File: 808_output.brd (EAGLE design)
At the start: 100.6 x 80.6 mm, 31 parts, among them IC1 TL072P

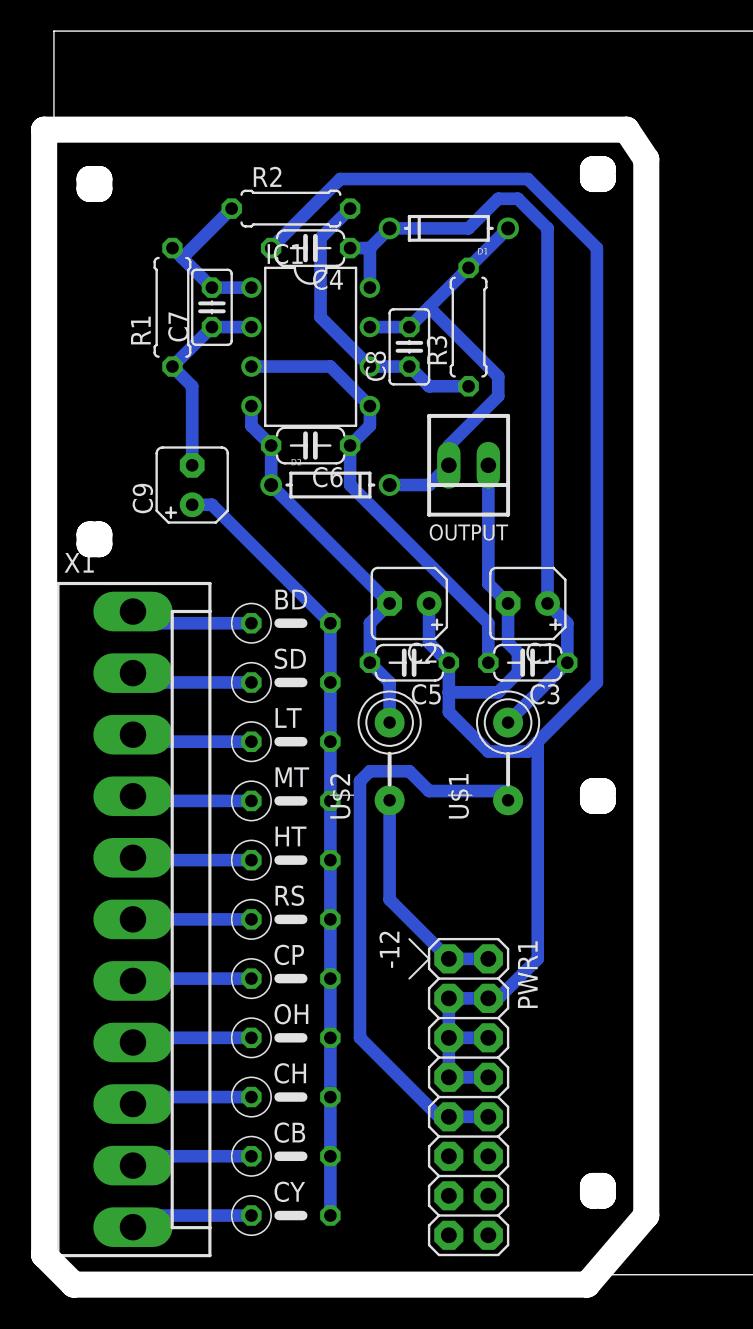
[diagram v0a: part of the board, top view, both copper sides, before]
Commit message: closer to og 808
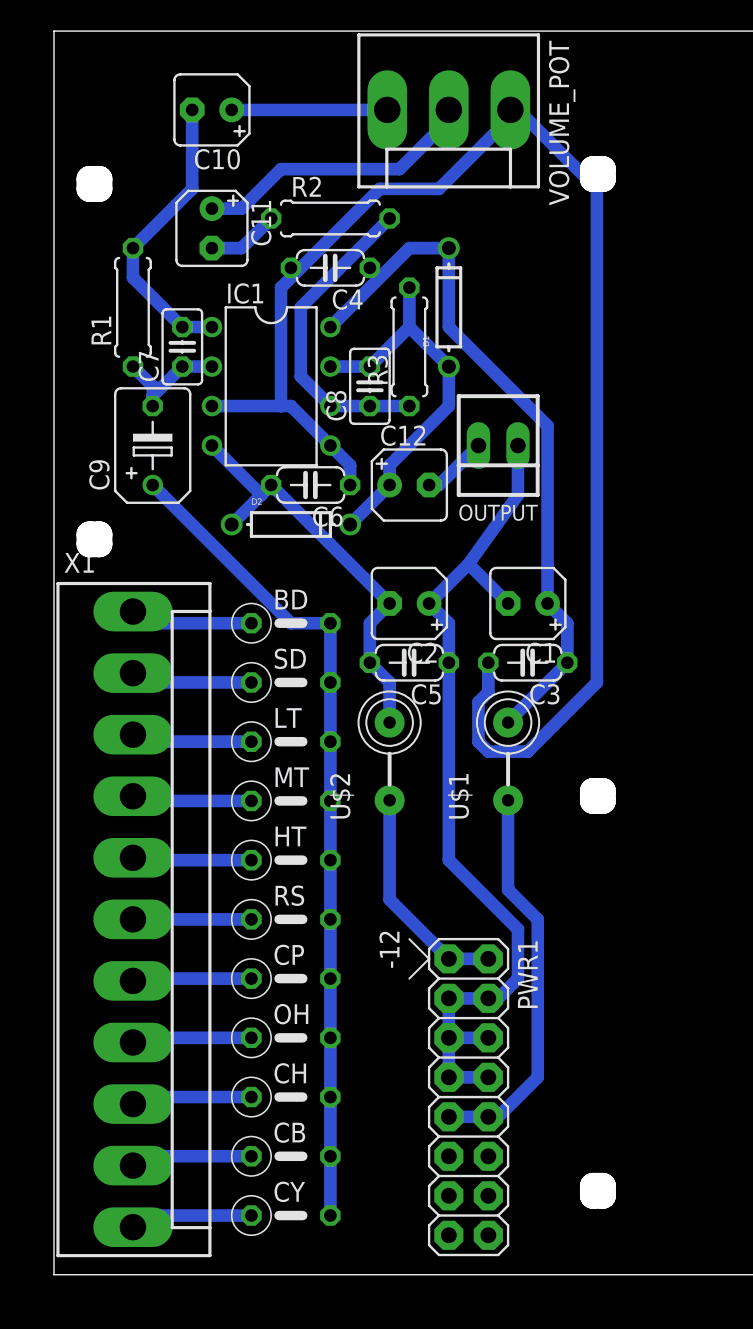
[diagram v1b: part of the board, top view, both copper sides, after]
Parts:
- added C10, C11: 1uF/50v, rcl:B45181A
- added C12: 10uF Bi, rcl:B45181A
- added VOLUME_POT: (no value), con-molex:KK-156-3
- C9: device rcl:B45181A -> rcl:B45181B
- moved D1 5.08 mm to (25.4, 62.2), turned to 90 degrees
- moved R3 4.02 mm to (22.9, 59.7)
- moved C9 3.59 mm to (6.35, 53.3)
- moved D2 3.59 mm to (15.2, 48.3)
- moved IC1 3.59 mm to (14.0, 57.1)
- moved C8 3.59 mm to (20.3, 57.1)
- moved C7 3.17 mm to (8.26, 59.7)
- moved R2 2.62 mm to (17.8, 67.9)
- moved C6 2.54 mm to (16.5, 50.8)
- moved R1 2.54 mm to (5.08, 62.2)
- moved OUTPUT 2.29 mm to (28.6, 53.3)
- moved C4 1.80 mm to (17.8, 64.8)
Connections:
- new net N$18: C11.-, R2.1
- new net N$20: C10.+, VOLUME_POT.3
- new net N$21: C11.+, VOLUME_POT.2
- new net N$22: C12.-, OUTPUT.2
- net GND: now also VOLUME_POT.1
- net N$15: now also C10.-; no longer R2.1
- net N$19: now also C12.+; no longer OUTPUT.2
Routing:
- net N$26: track 122.5 -> 57.4 mm
- net GND: track 29.4 -> 93.8 mm
- net N$21: track 0.00 -> 18.2 mm
- net N$1: track 37.8 -> 25.4 mm
- net N$20: track 0.00 -> 10.0 mm
- net N$15: track 10.6 -> 18.8 mm
- net +12V: track 51.2 -> 45.0 mm
- net N$17: track 13.0 -> 7.67 mm
- net N$18: track 0.00 -> 4.60 mm
- net N$22: track 0.00 -> 4.23 mm
- net N$19: track 29.2 -> 25.1 mm
- net N$14: track 50.1 -> 53.2 mm
- net -12V: track 25.1 -> 27.6 mm
- net N$16: track 19.1 -> 20.3 mm
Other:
- board size 100.6 x 80.6 mm -> 100 x 80 mm

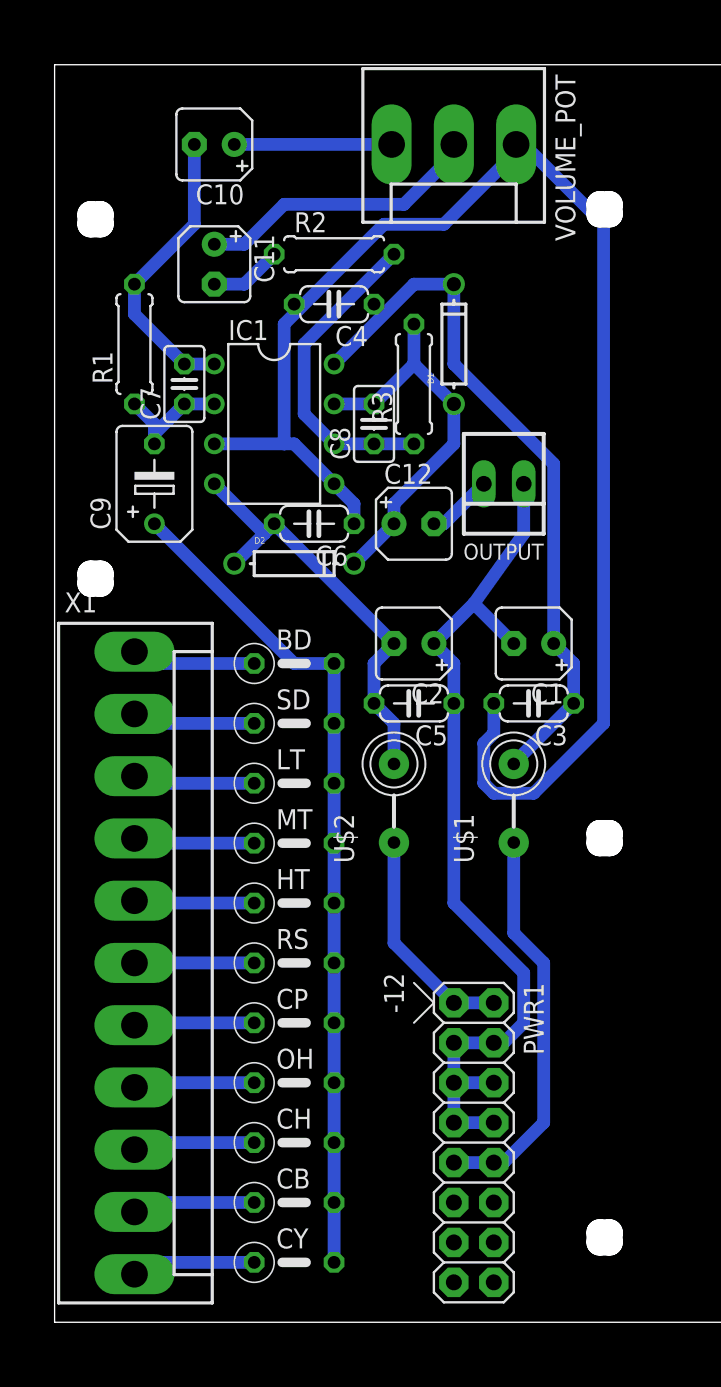
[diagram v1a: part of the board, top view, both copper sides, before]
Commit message: routed
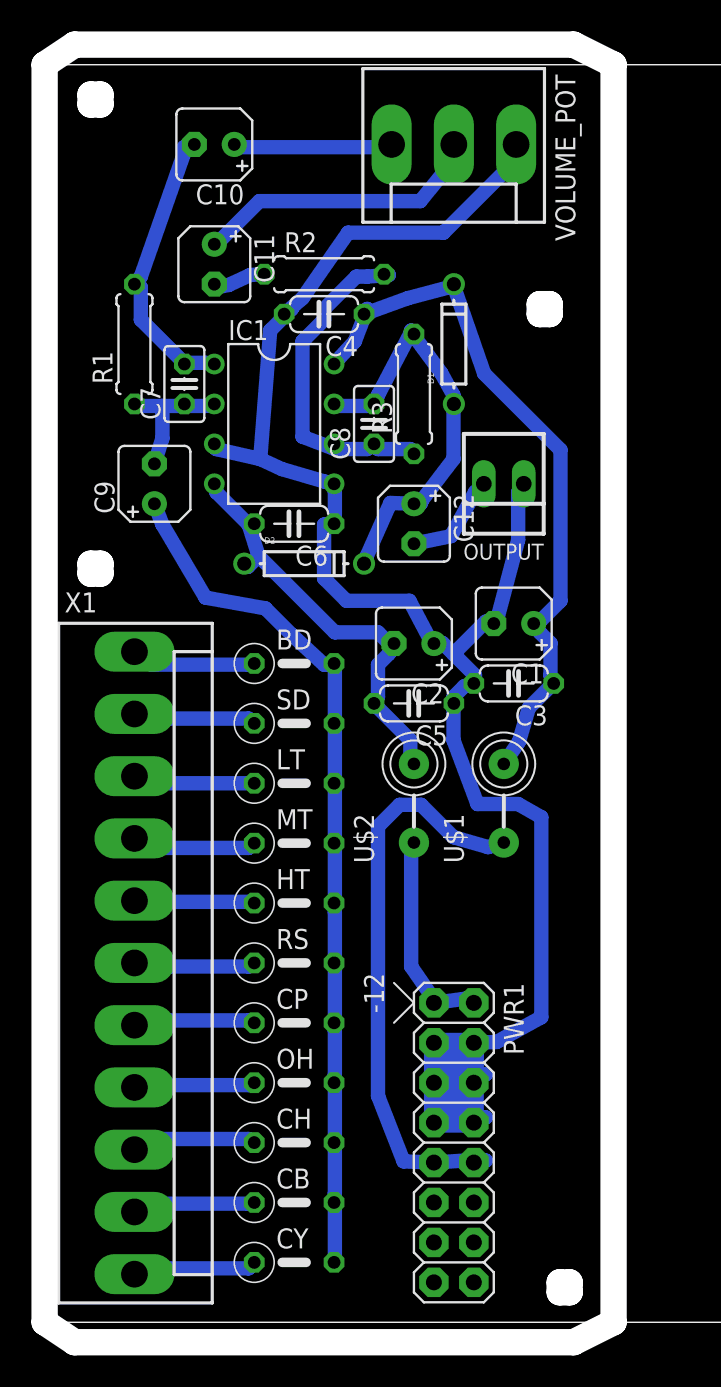
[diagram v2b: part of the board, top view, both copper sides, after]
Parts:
- C9: device rcl:B45181B -> rcl:B45181A
- moved C1 1.80 mm to (29.2, 44.5)
- moved C3 1.80 mm to (29.2, 40.6)
- moved R2 1.42 mm to (17.1, 66.7)
- moved PWR1 1.27 mm to (25.4, 14.0)
- moved C6 1.27 mm to (15.2, 50.8)
- moved U$2 1.27 mm to (22.9, 33.0)
- moved C4 0.90 mm to (17.1, 64.1)
- moved U$1 0.64 mm to (28.6, 33.0)
- moved D2 0.63 mm to (15.9, 48.3)
- moved R3 0.63 mm to (22.9, 59.1)
- turned C12 to 270 degrees
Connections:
- removed net N$26: C1.-, C2.+, C4.2, C5.1, OUTPUT.1, PWR1.3, PWR1.4, PWR1.5, PWR1.6, PWR1.7, PWR1.8
- net GND: now also C1.-, C2.+, C4.2, C5.1, OUTPUT.1, PWR1.3, PWR1.4, PWR1.5, PWR1.6, PWR1.7, PWR1.8
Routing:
- net N$26: track 57.4 -> 0.00 mm
- net GND: track 93.8 -> 118.6 mm
- net N$1: track 25.4 -> 37.2 mm
- net N$22: track 4.23 -> 6.37 mm
- net N$19: track 25.1 -> 26.8 mm
- net N$16: track 20.3 -> 22.0 mm
- net N$14: track 53.2 -> 54.8 mm
- net N$17: track 7.67 -> 9.00 mm
- net N$18: track 4.60 -> 3.44 mm
- net N$21: track 18.2 -> 19.3 mm
- net N$2: track 14.3 -> 13.3 mm
- net +12V: track 45.0 -> 45.9 mm
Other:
- board size 100 x 80 mm -> 100.6 x 82.5 mm
